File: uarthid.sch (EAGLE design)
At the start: 2 parts, among them IC1 FT230XQ, IC2 MEGA8-MI

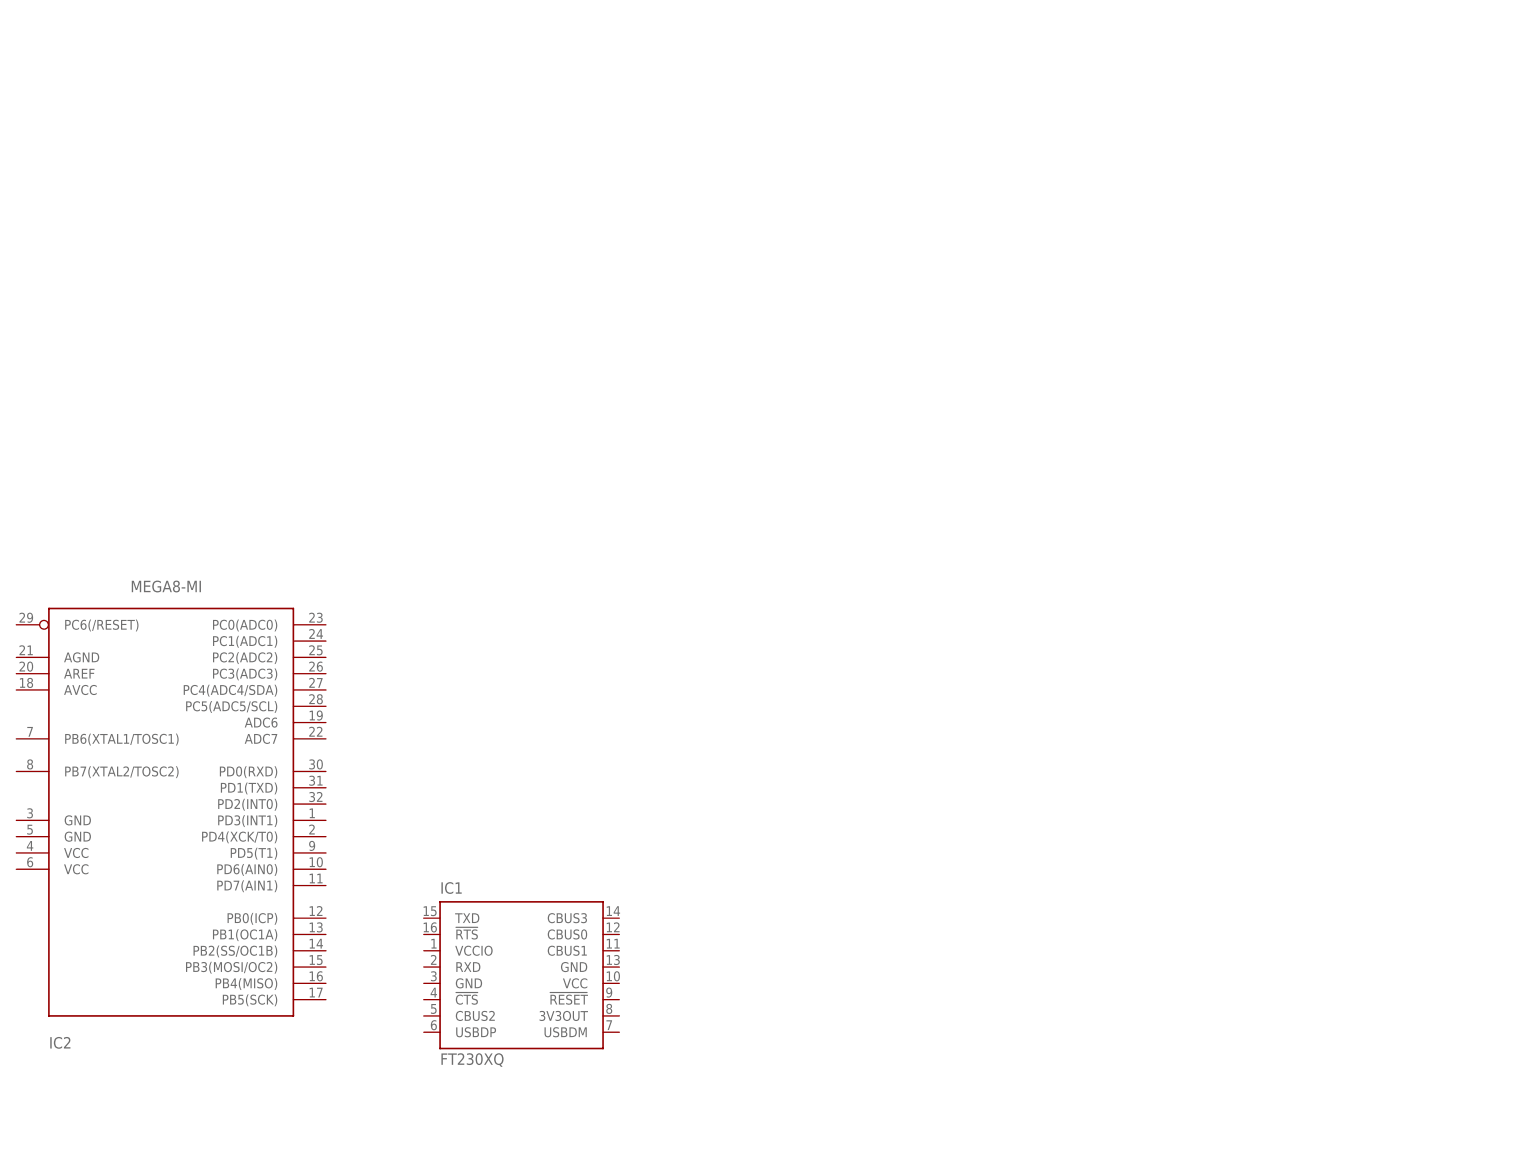
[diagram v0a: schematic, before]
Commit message: routed and bom'd
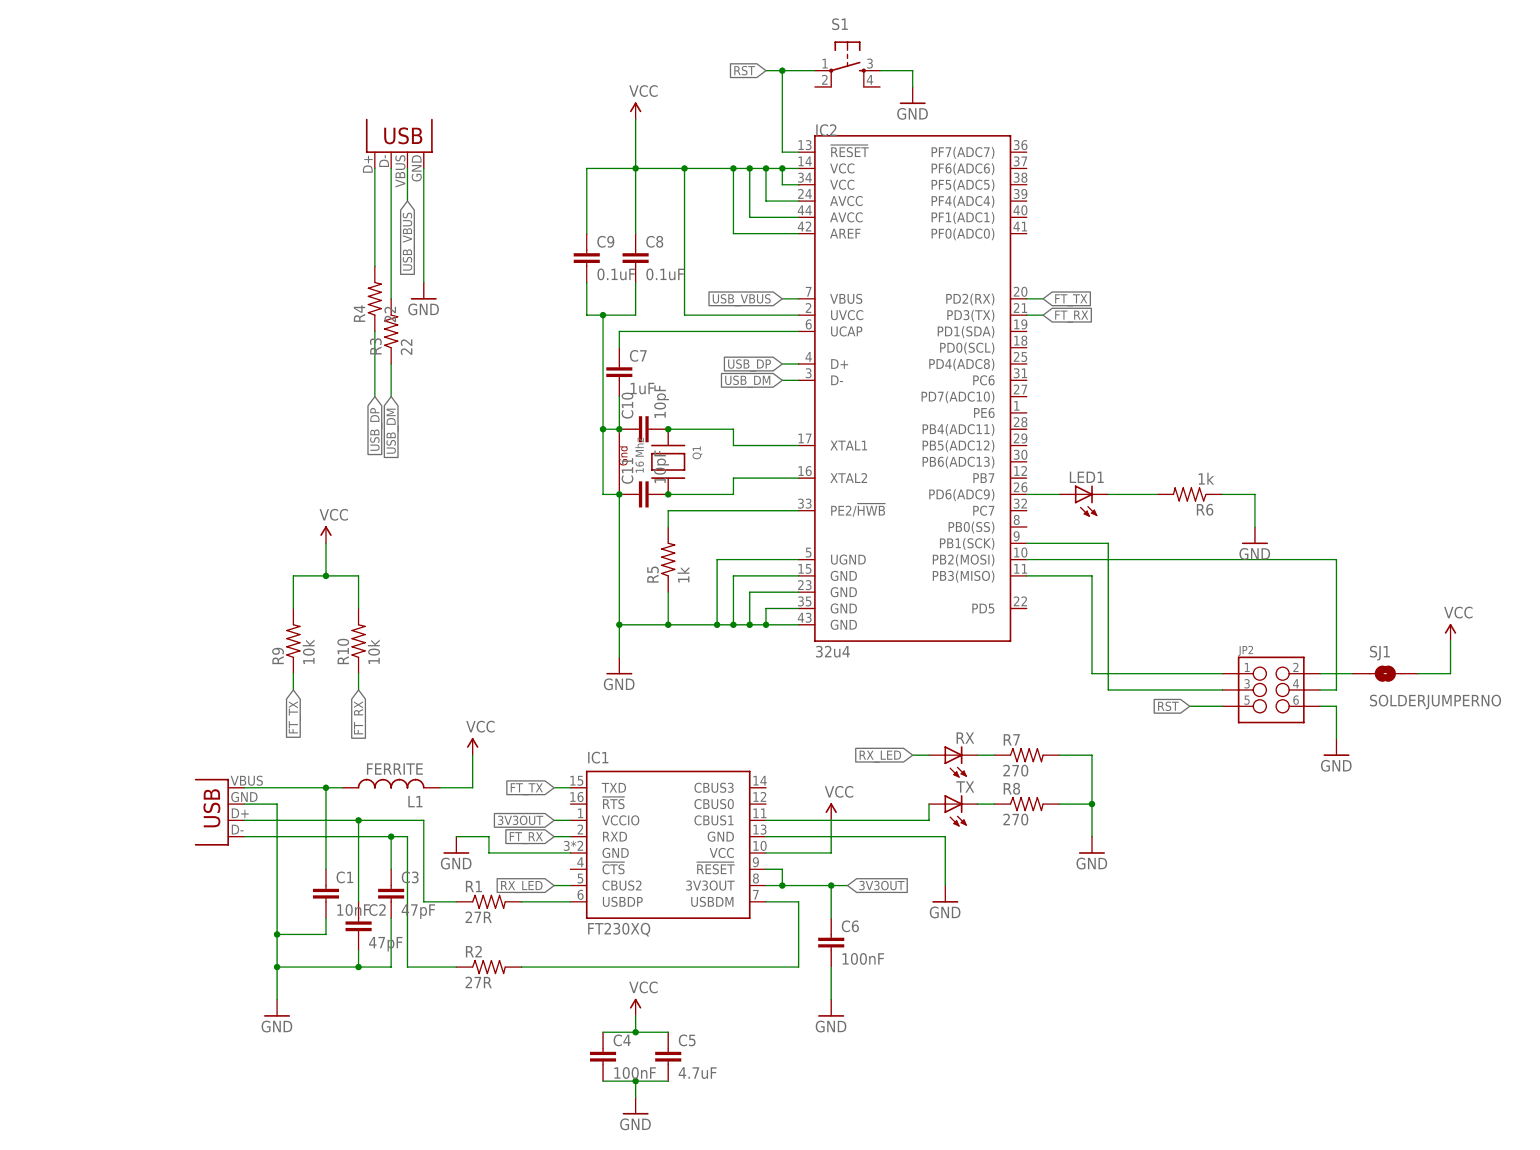
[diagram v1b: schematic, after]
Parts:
- added C1: 10nF, SparkFun-Capacitors:CAP0805
- added C10, C11: 10pF, SparkFun-Capacitors:CAP0805
- added C2, C3: 47pF, SparkFun-Capacitors:CAP0805
- added C4, C6: 100nF, SparkFun-Capacitors:CAP0805
- added C5: 4.7uF, SparkFun-Capacitors:CAP0805
- added C7: 1uF, SparkFun-Capacitors:CAP0805
- added C8, C9: 0.1uF, SparkFun-Capacitors:CAP0805
- added JP1: USB-A-H, SparkFun-Connectors:USB-A-H
- added JP2: (no value), SparkFun-Connectors:M03X22X3_SILK_SM
- added JP3: USBSMD, SparkFun-Connectors:USBSMD
- added L1: FERRITE, Livestream:FERRITE
- added LED1, RX, TX: (no value), adafruit:LEDCHIPLED_0805
- added Q1: 16 Mhz, adafruit:XTAL-4-3225
- added R1, R2: 27R, SparkFun-Passives:RESISTOR0805-RES
- added R10, R9: 10k, SparkFun-Passives:RESISTOR0805-RES
- added R3, R4: 22, SparkFun-Passives:RESISTOR0805-RES
- added R5, R6: 1k, SparkFun-Passives:RESISTOR0805-RES
- added R7, R8: 270, SparkFun-Passives:RESISTOR0805-RES
- added S1: (no value), SparkFun-Electromechanical:TAC_SWITCHSMD
- added SJ1: SOLDERJUMPERNO, SparkFun-Passives:SOLDERJUMPERNO
- IC1: PARTNO (none) -> FT230XQ-T
- IC2: value MEGA8-MI -> 32u4; device avr-5:MEGA8-MI -> SparkFun-DigitalIC:ATMEGA32U4QFN; PARTNO (none) -> ATMEGA32U4RC-MU
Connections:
- new net 3V3OUT: C6.1, IC1.!RESET, IC1.3V3OUT, IC1.VCCIO
- new net FT_RX: IC1.RXD, IC2.PD3(TX), R10.1
- new net FT_TX: IC1.TXD, IC2.PD2(RX), R9.1
- new net GND: C1.2, C10.1, C11.1, C2.2, C3.2, C4.2, C5.2, C6.2, C7.2, C8.2, C9.2, IC1.GND, IC1.GND@1, IC2.GND@15, IC2.GND@23, IC2.GND@35, IC2.GND@43, IC2.UGND, JP1.VBUS, JP2.6, JP3.GND, Q1.G1, Q1.G2, R5.1, R6.1, R7.2, R8.2, S1.3
- new net N$1: C2.1, JP1.D-, R1.1
- new net N$10: JP2.2, SJ1.1
- new net N$11: C7.1, IC2.UCAP
- new net N$12: IC2.PB3(MISO), JP2.1
- new net N$13: IC2.PB1(SCK), JP2.3
- new net N$14: IC2.PB2(MOSI), JP2.4
- new net N$15: IC2.PE2/!HWB, R5.2
- new net N$16: IC2.PD6(ADC9), LED1.A
- new net N$17: LED1.C, R6.2
- new net N$18: IC1.CBUS1, TX.A
- new net N$19: R7.1, RX.C
- new net N$2: IC1.USBDP, R1.2
- new net N$20: R8.1, TX.C
- new net N$3: C3.1, JP1.D+, R2.1
- new net N$4: IC1.USBDM, R2.2
- new net N$5: C1.1, JP1.GND, L1.1
- new net N$6: C10.2, IC2.XTAL1, Q1.X1
- new net N$7: C11.2, IC2.XTAL2, Q1.X2
- new net N$8: JP3.D-, R3.2
- new net N$9: JP3.D+, R4.2
- new net RST: IC2.!RESET, JP2.5, S1.1
- new net RX_LED: IC1.CBUS2, RX.A
- new net USB_DM: IC2.D-, R3.1
- new net USB_DP: IC2.D+, R4.1
- new net USB_VBUS: IC2.VBUS, JP3.VBUS
- new net VCC: C4.1, C5.1, C8.1, C9.1, IC1.VCC, IC2.AREF, IC2.AVCC@24, IC2.AVCC@44, IC2.UVCC, IC2.VCC@14, IC2.VCC@34, L1.2, R10.2, R9.2, SJ1.2
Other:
- moved on the sheet: IC1
